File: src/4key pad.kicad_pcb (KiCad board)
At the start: 2 copper layers, 78 x 39 mm, 7 parts, among them J1 OLED_128x32, SW1 RotaryEncoder_Switch_MP, U2 Raspberry_Pi_Pico

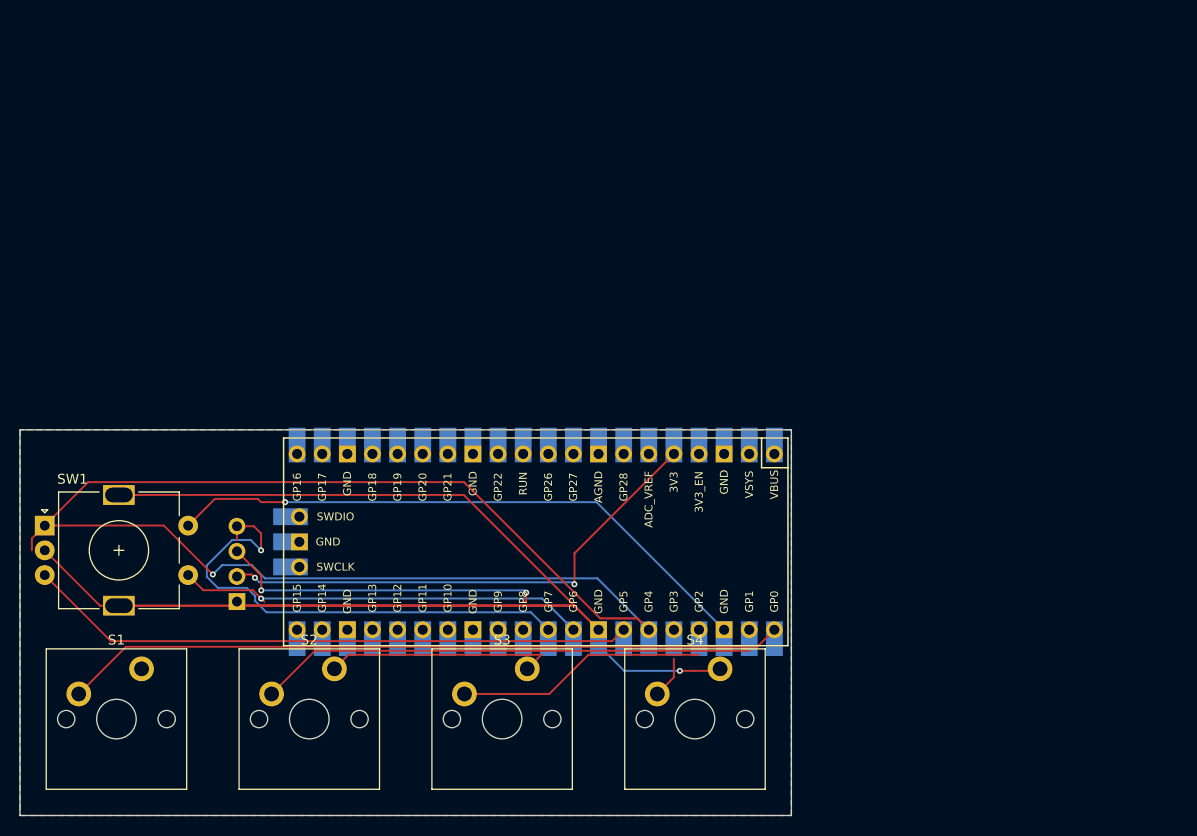
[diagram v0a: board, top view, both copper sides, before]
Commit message: Add files via upload
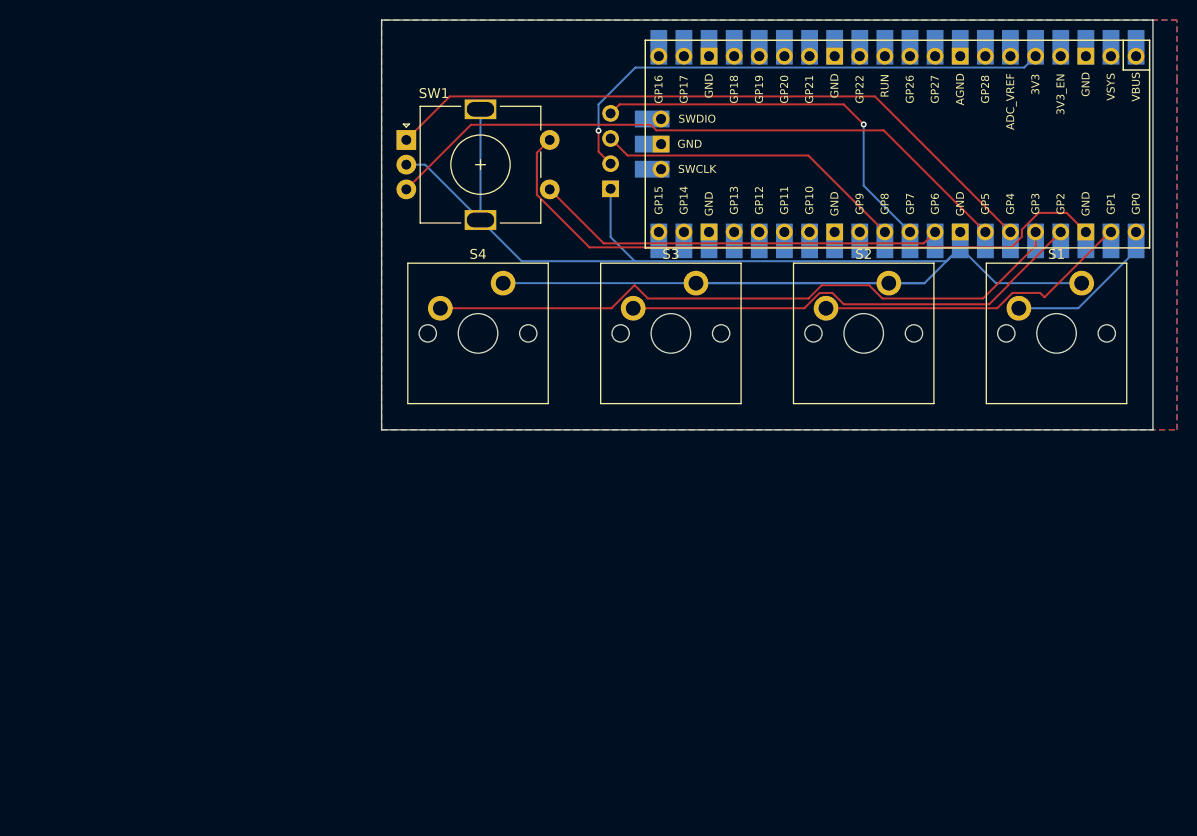
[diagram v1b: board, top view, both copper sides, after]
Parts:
- moved S1 102.8 mm to (226.7, 43.9)
- moved S2 68.3 mm to (207.2, 43.9)
- moved J1 56.3 mm to (180.0, 19.4)
- moved U2 54.4 mm to (210.6, 24.7)
- moved SW1 53.5 mm to (160.9, 24.3)
- moved S4 44.7 mm to (168.2, 43.9)
- moved S3 42.6 mm to (187.7, 43.9)
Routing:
- net swa: track 138.4 -> 68.6 mm, vias 1 -> 0
- net GND: track 232.4 -> 169.9 mm, vias 1 -> 0
- net sw4: track 4.27 -> 66.4 mm
- net sw1: track 73.0 -> 16.1 mm
- net sw3: track 25.4 -> 47.4 mm
- net sw2: track 50.1 -> 32.4 mm
- net sda: track 51.0 -> 39.6 mm
- net rsw2: track 60.8 -> 66.5 mm, vias 1 -> 0
- net swb: track 61.8 -> 65.7 mm
- net scl: track 33.1 -> 31.7 mm, vias 2 -> 0
- net VCC: track 52.1 -> 52.7 mm, vias 2 -> 1
- net rsw1: vias 1 -> 0
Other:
- board size 78 x 39 mm -> 78 x 41.4 mm
